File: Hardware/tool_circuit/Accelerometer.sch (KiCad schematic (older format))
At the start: 1 part, among them J3 Conn_01x08_Female

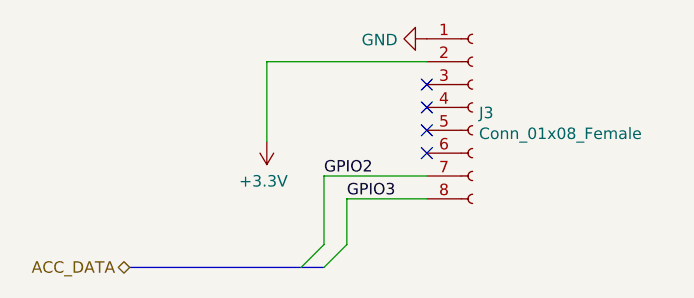
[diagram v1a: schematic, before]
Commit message: pcb revisions
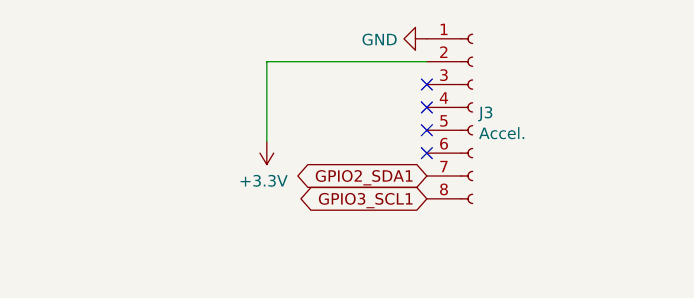
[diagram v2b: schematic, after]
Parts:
- J3: value Conn_01x08_Female -> Accel.
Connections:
- net GPIO2 renamed GPIO2_SDA1
- net GPIO3 renamed GPIO3_SCL1
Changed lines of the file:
@@
 $Descr A4 11693 8268
 encoding utf-8
-Sheet 7 8
+Sheet 8 8
 Title "Accelerometer "
 Date ""
@@
 Comment4 ""
 $EndDescr
-Wire Wire Line
-	5550 4200 5550 3900
-Wire Wire Line
-	5650 4200 5650 4000
-Text Label 5550 3900 0    50   ~ 0
-GPIO2
-Text Label 5650 4000 0    50   ~ 0
-GPIO3
-Text HLabel 4700 4300 0    50   BiDi ~ 0
-ACC_DATA
-Entry Wire Line
-	5550 4300 5650 4200
-Entry Wire Line
-	5450 4300 5550 4200
 $Comp
 L Connector:Conn_01x08_Female J3
@@
 P 6200 3600
 F 0 "J3" H 6228 3576 50  0000 L CNN
-F 1 "Conn_01x08_Female" H 6228 3485 50  0000 L CNN
+F 1 "Accel." H 6228 3485 50  0000 L CNN
 F 2 "Connector_PinHeader_2.54mm:PinHeader_1x08_P2.54mm_Vertical" H 6200 3600 50  0001 C CNN
 F 3 "~" H 6200 3600 50  0001 C CNN
@@
 	1    0    0    -1
 $EndComp
-Wire Wire Line
-	5650 4000 6000 4000
 Wire Wire Line
 	5300 3400 6000 3400
@@
 NoConn ~ 6000 3700
 NoConn ~ 6000 3800
-Wire Wire Line
-	5550 3900 6000 3900
 $Comp
 L power:GND #PWR011
@@
 	0    1    1    0
 $EndComp
-Wire Bus Line
-	4700 4300 5550 4300
+Text GLabel 6000 3900 0    50   BiDi ~ 0
+GPIO2_SDA1
+Text GLabel 6000 4000 0    50   BiDi ~ 0
+GPIO3_SCL1
 $EndSCHEMATC
